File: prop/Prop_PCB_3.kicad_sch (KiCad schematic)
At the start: 25 parts

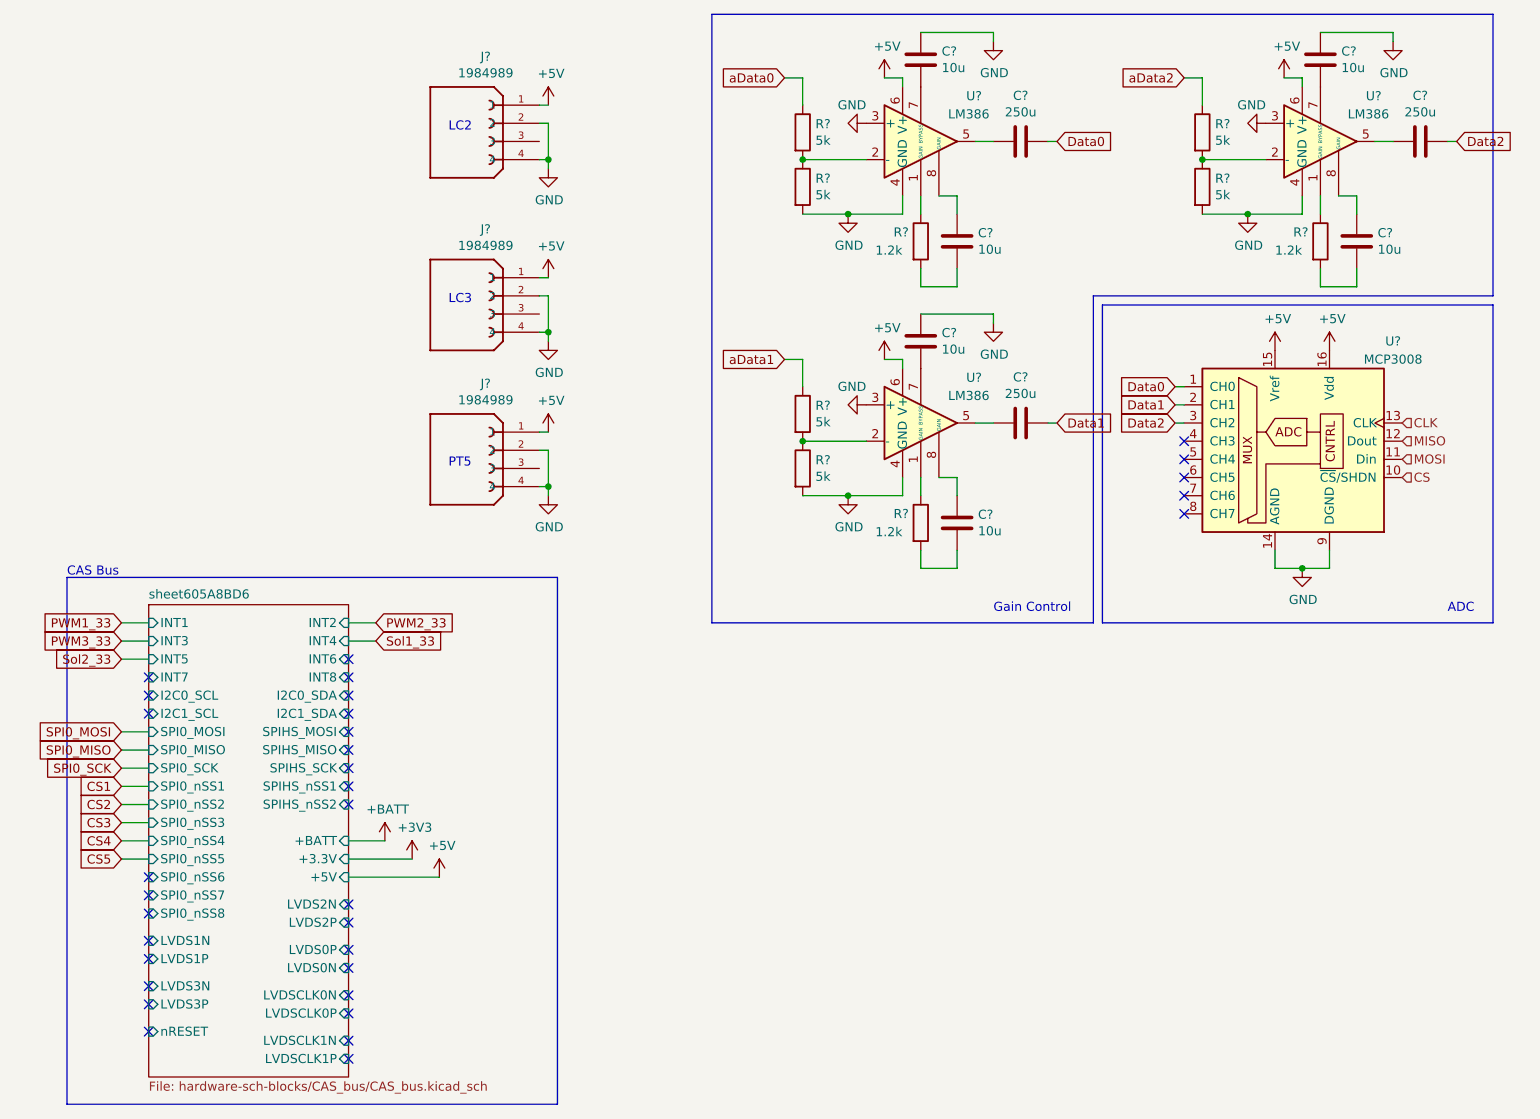
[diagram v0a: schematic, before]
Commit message: finalize3pcb schematic
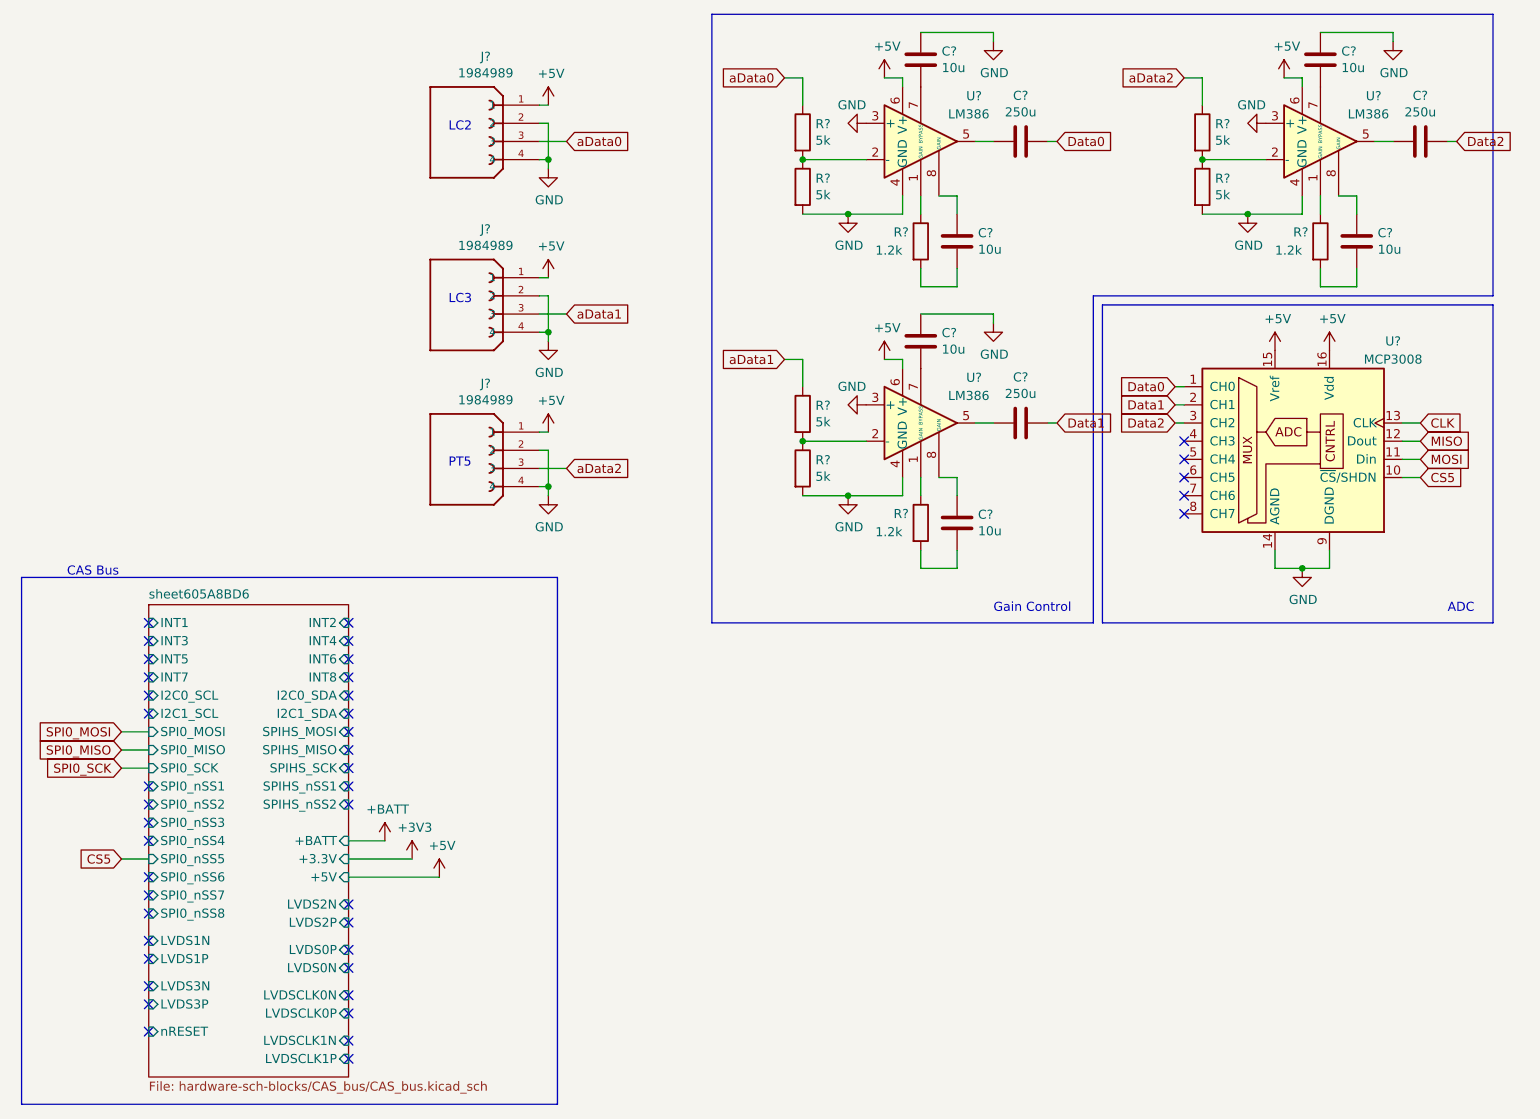
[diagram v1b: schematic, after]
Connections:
- net CS is gone; now on net CS5: U?.10 (~{CS}/SHDN)
- net aData0: now also J?.3
- net aData1: now also J?.3
- net aData2: now also J?.3
- no-connect marks 33 -> 42
